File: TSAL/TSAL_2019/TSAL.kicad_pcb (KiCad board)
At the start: 2 copper layers, 68.6 x 68.6 mm, 101 parts, among them J1 Main Connector, Q1 TSM320N03CX, Q2 TSM320N03CX, Q3 TSM320N03CX, Q4 TSM320N03CX, U1 SE555

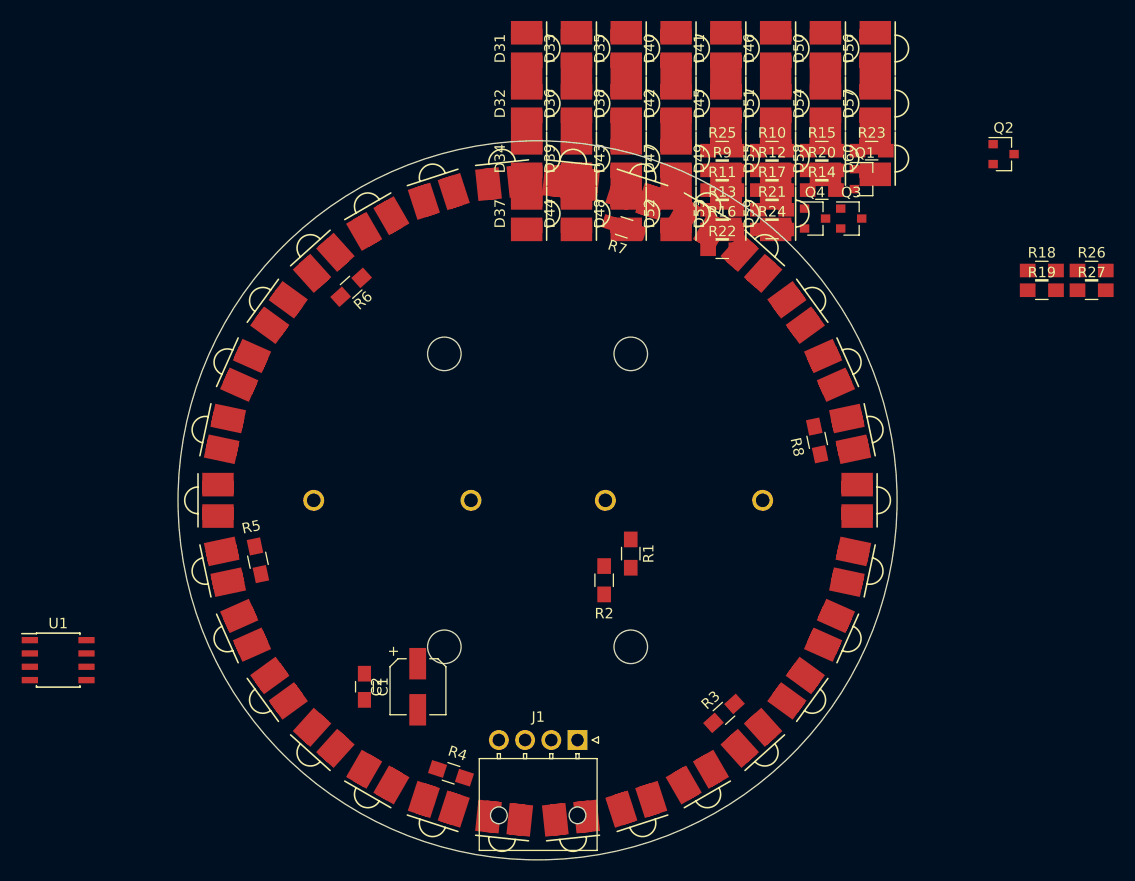
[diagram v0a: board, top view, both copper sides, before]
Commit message: Finish layout of TSAL 2019 (ugly edition)
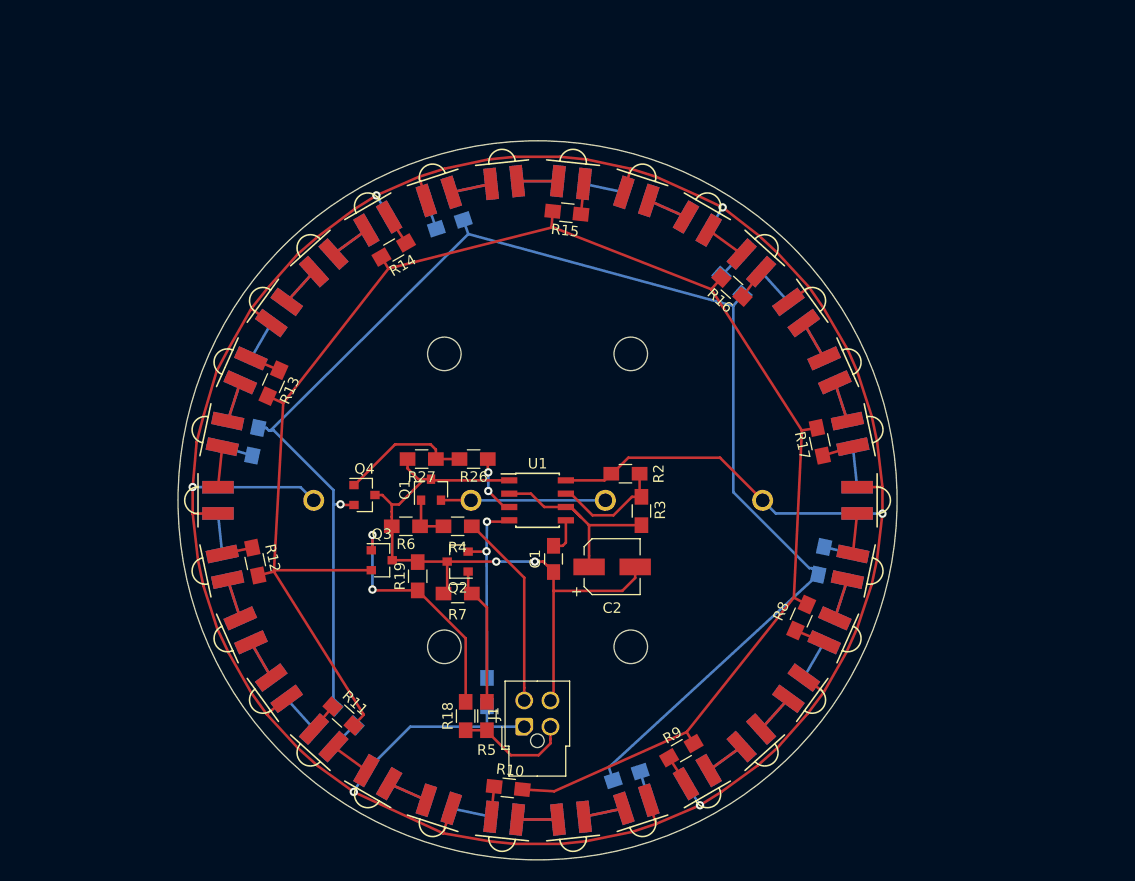
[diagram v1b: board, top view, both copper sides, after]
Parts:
- D31, D32, D33, D34, D35, D36, D37, D38, D39, D40, D41, D42, D43, D44, D45, D46, D47, D48, D49, D50, D51, D52, D53, D54, D55, D56, D57, D58, D59, D60, R1, R20, R21, R22, R23, R24, R25: moved to B.Cu
- J1: footprint Connectors_Molex:Molex_NanoFit_1x04x2.50mm_Angled -> Connector_Molex:Molex_Nano-Fit_105310-xx04_2x02_P2.50mm_Vertical
- moved D50 81.3 mm to (132.0, 124.3), turned to 228 degrees
- moved D51 74.6 mm to (137.2, 128.0), turned to 240 degrees
- moved R23 73.8 mm to (133.9, 122.2), turned to 138 degrees
- moved D54 72.4 mm to (155.6, 131.9), turned to 276 degrees
- moved D56 71.5 mm to (167.6, 128.0), turned to 300 degrees
- moved R18 69.5 mm to (145.5, 122.2), turned to 90 degrees
- moved D46 68.5 mm to (121.9, 101.6), turned to 180 degrees
- moved D49 66.1 mm to (127.7, 119.5), turned to 216 degrees
- moved R27 65.9 mm to (141.4, 97.7), turned to 180 degrees
- moved R10 65.8 mm to (149.6, 129.0), turned to 354 degrees
- moved R19 65.5 mm to (141.0, 108.8), turned to 90 degrees
- moved Q2 65.0 mm to (144.8, 107.4), turned to 180 degrees
- moved D55 63.0 mm to (161.8, 130.6), turned to 288 degrees
- moved R11 61.8 mm to (133.9, 122.2), turned to 318 degrees
- moved R12 61.8 mm to (125.5, 107.4), turned to 282 degrees
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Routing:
- net +12V: track 0.00 -> 305.1 mm, vias 0 -> 6
- net Net-(Q3-Pad2): track 0.00 -> 168.6 mm
- net Net-(Q4-Pad2): track 0.00 -> 145.4 mm, vias 0 -> 1
- net GND: track 0.00 -> 64.2 mm, vias 0 -> 2
- net Net-(Q3-Pad1): track 0.00 -> 23.6 mm, vias 0 -> 2
- net Net-(C2-Pad1): track 0.00 -> 19.2 mm
- net Net-(Q2-Pad2): track 0.00 -> 19.0 mm, vias 0 -> 2
- net SIG_RTDS: track 0.00 -> 18.7 mm
- net Net-(LS1-Pad2): track 0.00 -> 15.7 mm
- net Net-(Q2-Pad1): track 0.00 -> 13.2 mm
- net Net-(Q4-Pad1): track 0.00 -> 12.8 mm
- net SIG_TSAL: track 0.00 -> 11.2 mm
- net Net-(R2-Pad2): track 0.00 -> 11.2 mm
- net 555: track 0.00 -> 5.70 mm, vias 0 -> 2
- net Net-(Q1-Pad1): track 0.00 -> 4.77 mm
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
